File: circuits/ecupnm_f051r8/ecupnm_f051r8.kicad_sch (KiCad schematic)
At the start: 57 parts, among them J1 Conn_01x03_Pin, J2 Conn_01x03_Pin, J3 Conn_01x05_Pin, J4 Conn_01x03_Pin, J5 USB_B_Mini, U1 STM32F051R8Tx, U6 AMS1117-5.0, U7 AMS1117-3.3

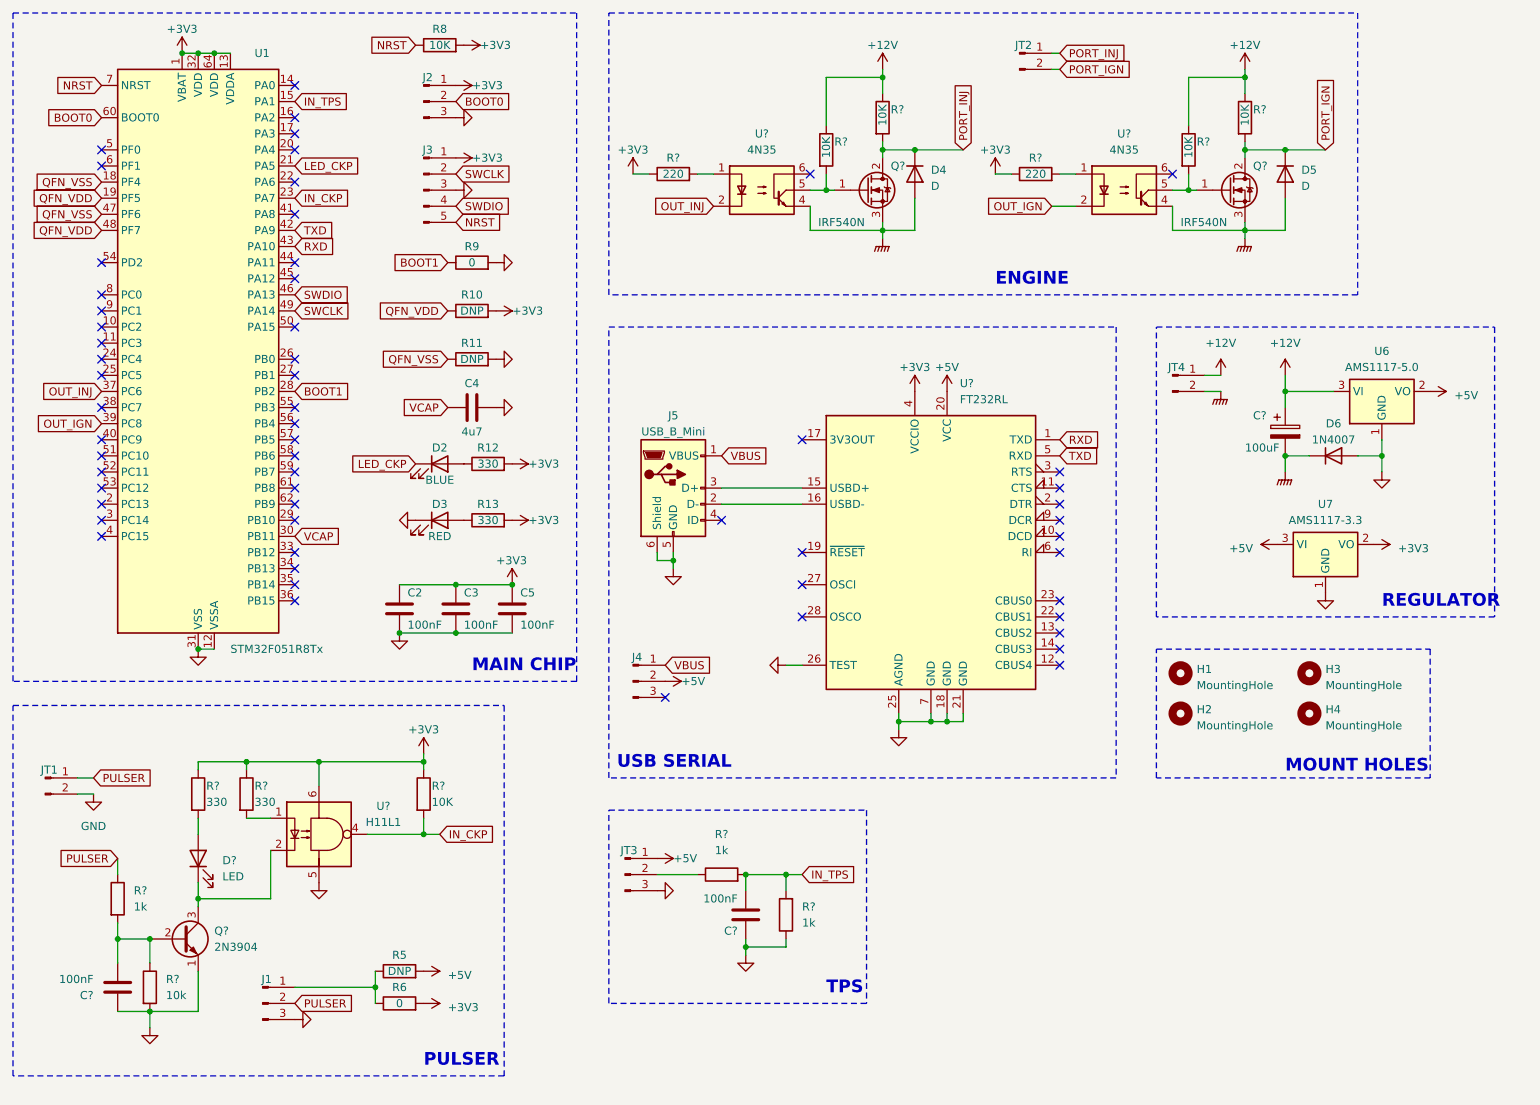
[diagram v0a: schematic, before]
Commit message: New PCB
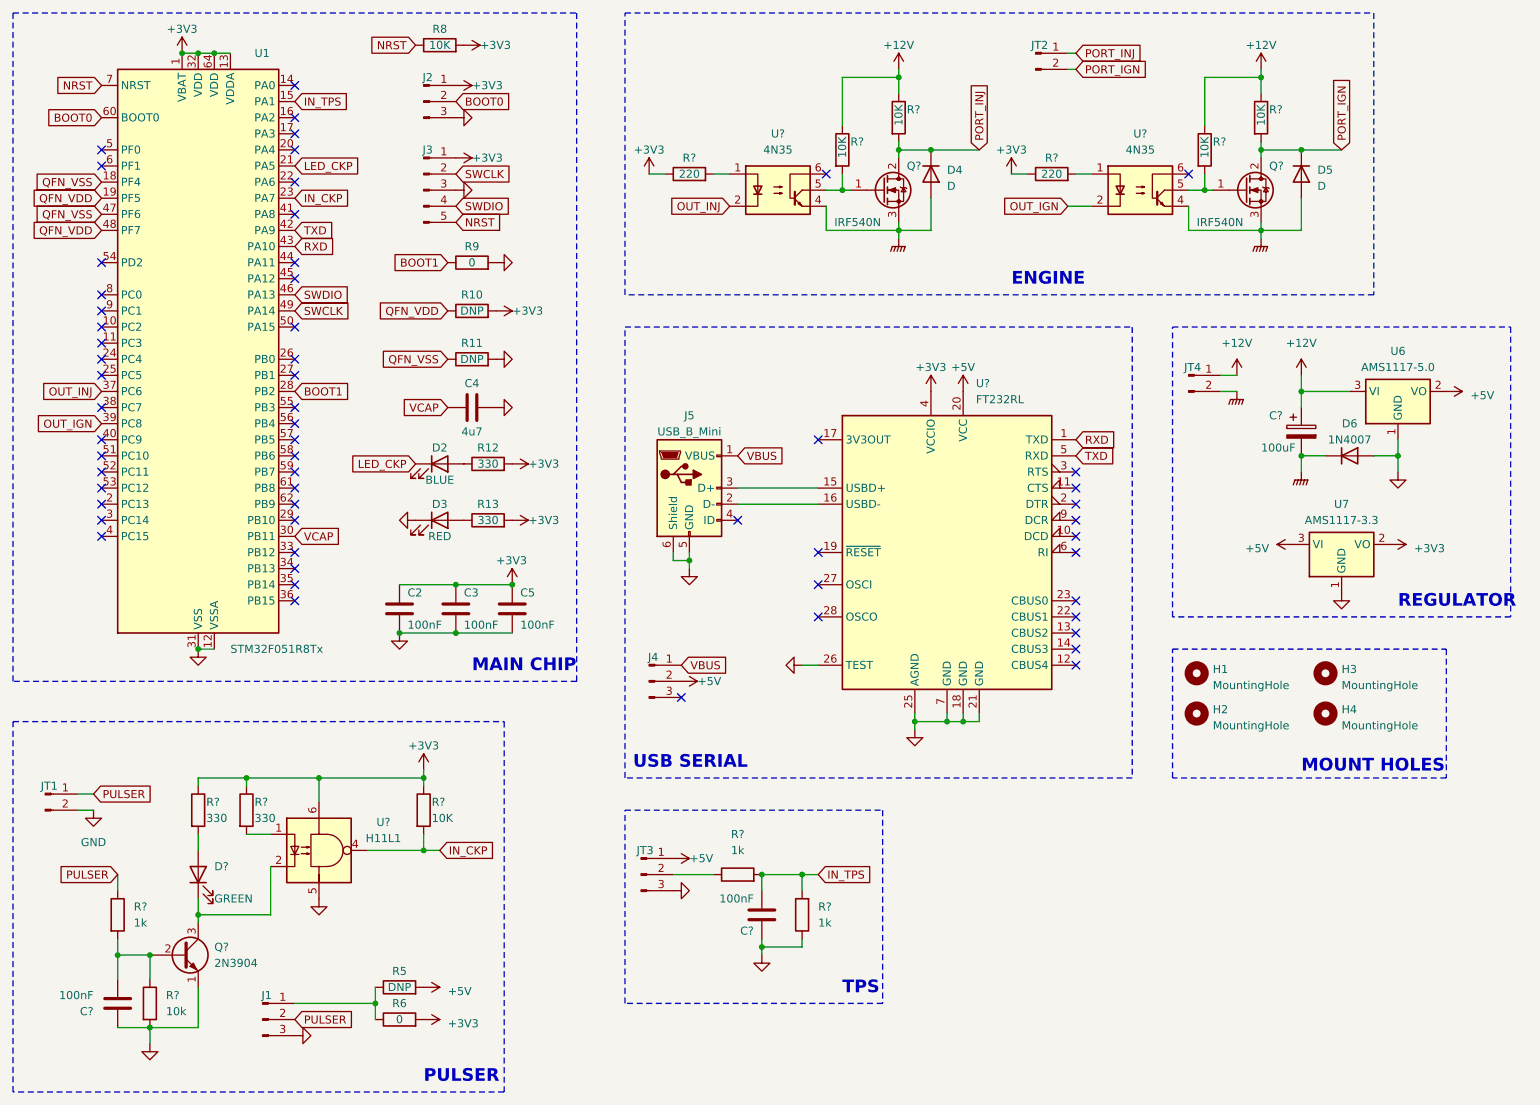
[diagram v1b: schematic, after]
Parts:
- C2, C3, C4, C5: footprint (none) -> Capacitor_SMD:C_0805_2012Metric_Pad1.18x1.45mm_HandSolder
- C? (x2): footprint Capacitor_SMD:C_1206_3216Metric_Pad1.33x1.80mm_HandSolder -> Capacitor_SMD:C_0805_2012Metric_Pad1.18x1.45mm_HandSolder
- D2, D3: footprint (none) -> LED_SMD:LED_0805_2012Metric_Pad1.15x1.40mm_HandSolder
- D?: value LED -> GREEN; footprint LED_SMD:LED_1206_3216Metric_Pad1.42x1.75mm_HandSolder -> LED_SMD:LED_0805_2012Metric_Pad1.15x1.40mm_HandSolder
- J2, J4: footprint (none) -> Connector_PinHeader_2.54mm:PinHeader_1x03_P2.54mm_Vertical
- J3: footprint (none) -> Connector_PinHeader_2.54mm:PinHeader_1x05_P2.54mm_Vertical
- R10, R11, R12, R13, R5, R6, R8, R9: footprint (none) -> Resistor_SMD:R_0805_2012Metric_Pad1.20x1.40mm_HandSolder
- R? (x13): footprint Resistor_SMD:R_1206_3216Metric_Pad1.30x1.75mm_HandSolder -> Resistor_SMD:R_0805_2012Metric_Pad1.20x1.40mm_HandSolder
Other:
- company: (none) -> Politeknik Negeri Madiun
- title: (none) -> Custom Engine Control
- moved on the sheet: C?, D4, D5, D6, D?, H1, H2, H3, H4, J1, J4, J5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

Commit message: PCB Baru
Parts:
- C?: footprint Capacitor_THT:CP_Radial_D7.5mm_P2.50mm -> Capacitor_THT:CP_Radial_D4.0mm_P2.00mm
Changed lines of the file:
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@@
       (effects (font (size 1.27 1.27)) (justify left))
     )
-    (property "Footprint" "Capacitor_THT:CP_Radial_D7.5mm_P2.50mm" (at 239.7252 90.17 0)
+    (property "Footprint" "Capacitor_THT:CP_Radial_D4.0mm_P2.00mm" (at 239.7252 90.17 0)
       (effects (font (size 1.27 1.27)) hide)
     )

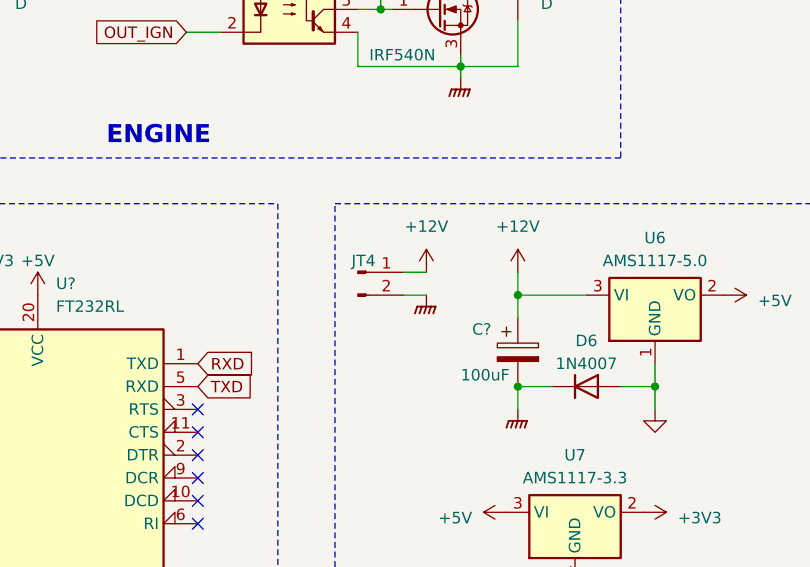
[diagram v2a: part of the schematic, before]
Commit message: Mulai Order
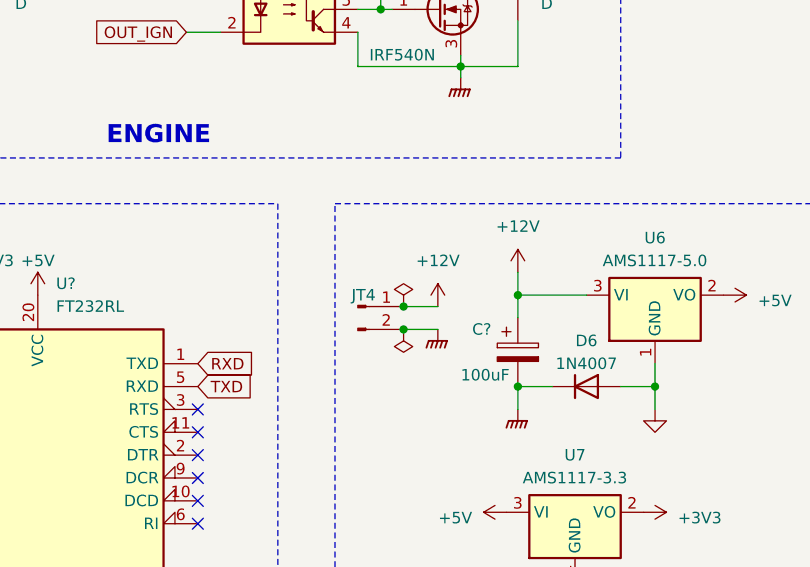
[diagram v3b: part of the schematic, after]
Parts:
- Q? (x2): footprint Package_TO_SOT_THT:TO-220-3_Horizontal_TabDown -> Package_TO_SOT_THT:TO-220-3_Vertical
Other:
- moved on the sheet: JT4
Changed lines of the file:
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@@
   (junction (at 177.8 132.08) (diameter 0) (color 0 0 0 0)
   )
+  (junction (at 226.06 81.28) (diameter 0) (color 0 0 0 0)
+  )
   (junction (at 72.39 140.97) (diameter 0) (color 0 0 0 0)
   )
@@
   (junction (at 96.52 118.11) (diameter 0) (color 0 0 0 0)
   )
+  (junction (at 226.06 83.82) (diameter 0) (color 0 0 0 0)
+  )
   (junction (at 153.67 167.64) (diameter 0) (color 0 0 0 0)
   )
@@
     (stroke (width 0) (type default))
   )
-  (wire (pts (xy 226.06 77.47) (xy 228.6 77.47))
+  (wire (pts (xy 226.06 81.28) (xy 229.87 81.28))
     (stroke (width 0) (type default))
   )
@@
     (stroke (width 0) (type default))
   )
-  (wire (pts (xy 226.06 80.01) (xy 228.6 80.01))
+  (wire (pts (xy 226.06 83.82) (xy 229.87 83.82))
     (stroke (width 0) (type default))
   )
@@
     )
   )
-  (symbol (lib_id "Connector:Conn_01x02_Pin") (at 220.98 77.47 0) (unit 1)
+  (symbol (lib_id "Connector:Conn_01x02_Pin") (at 220.98 81.28 0) (unit 1)
     (in_bom yes) (on_board yes) (dnp no) (fields_autoplaced)
-    (property "Reference" "JT4" (at 221.615 76.2 0)
+    (property "Reference" "JT4" (at 221.615 80.01 0)
       (effects (font (size 1.27 1.27)))
     )
-    (property "Value" "Conn_01x02_Pin" (at 221.615 76.2 0)
+    (property "Value" "Conn_01x02_Pin" (at 221.615 80.01 0)
       (effects (font (size 1.27 1.27)) hide)
     )
-    (property "Footprint" "TerminalBlock:TerminalBlock_Altech_AK300-2_P5.00mm" (at 220.98 77.47 0)
+    (property "Footprint" "TerminalBlock:TerminalBlock_Altech_AK300-2_P5.00mm" (at 220.98 81.28 0)
       (effects (font (size 1.27 1.27)) hide)
     )
-    (property "Datasheet" "~" (at 220.98 77.47 0)
+    (property "Datasheet" "~" (at 220.98 81.28 0)
       (effects (font (size 1.27 1.27)) hide)
     )
@@
       (effects (font (size 1.27 1.27)) (justify left))
     )
-    (property "Footprint" "Package_TO_SOT_THT:TO-220-3_Horizontal_TabDown" (at 179.07 50.165 0)
+    (property "Footprint" "Package_TO_SOT_THT:TO-220-3_Vertical" (at 179.07 50.165 0)
       (effects (font (size 1.27 1.27) italic) (justify left) hide)
     )
@@
     )
   )
-  (symbol (lib_id "power:+12V") (at 228.6 77.47 0) (unit 1)
+  (symbol (lib_id "power:+12V") (at 229.87 81.28 0) (unit 1)
     (in_bom yes) (on_board yes) (dnp no) (fields_autoplaced)
-    (property "Reference" "#PWR?" (at 228.6 81.28 0)
+    (property "Reference" "#PWR?" (at 229.87 85.09 0)
       (effects (font (size 1.27 1.27)) hide)
     )
-    (property "Value" "+12V" (at 228.6 72.39 0)
+    (property "Value" "+12V" (at 229.87 76.2 0)
       (effects (font (size 1.27 1.27)))
     )
-    (property "Footprint" "" (at 228.6 77.47 0)
+    (property "Footprint" "" (at 229.87 81.28 0)
       (effects (font (size 1.27 1.27)) hide)
     )
-    (property "Datasheet" "" (at 228.6 77.47 0)
+    (property "Datasheet" "" (at 229.87 81.28 0)
       (effects (font (size 1.27 1.27)) hide)
     )
@@
     )
   )
-  (symbol (lib_name "+12V_1") (lib_id "power:+12V") (at 175.26 29.21 0) (unit 1)
+  (symbol (lib_id "power:PWR_FLAG") (at 226.06 81.28 0) (unit 1)
+    (in_bom yes) (on_board yes) (dnp no) (fields_autoplaced)
+    (property "Reference" "#FLG01" (at 226.06 79.375 0)
+      (effects (font (size 1.27 1.27)) hide)
+    )
+    (property "Value" "PWR_FLAG" (at 226.06 77.47 0)
+      (effects (font (size 1.27 1.27)) hide)
+    )
+    (property "Footprint" "" (at 226.06 81.28 0)
+      (effects (font (size 1.27 1.27)) hide)
+    )
+    (property "Datasheet" "~" (at 226.06 81.28 0)
+      (effects (font (size 1.27 1.27)) hide)
+    )
+    (pin "1")
+    (instances
+      (project "ecupnm_f051r8"
+        (path "/6d87dde5-b75c-4573-a03b-3b31eef01557"
+          (reference "#FLG01") (unit 1)
+        )
+      )
+    )
+  )
+  (symbol (lib_id "power:+12V") (at 175.26 29.21 0) (unit 1)
     (in_bom yes) (on_board yes) (dnp no)
     (property "Reference" "#PWR028" (at 175.26 33.02 0)
@@
     )
   )
-  (symbol (lib_id "power:GNDPWR") (at 228.6 80.01 0) (unit 1)
+  (symbol (lib_id "power:GNDPWR") (at 229.87 83.82 0) (unit 1)
     (in_bom yes) (on_board yes) (dnp no) (fields_autoplaced)
-    (property "Reference" "#PWR?" (at 228.6 85.09 0)
+    (property "Reference" "#PWR?" (at 229.87 88.9 0)
       (effects (font (size 1.27 1.27)) hide)
     )
-    (property "Value" "GNDPWR" (at 228.473 85.09 0)
+    (property "Value" "GNDPWR" (at 229.743 88.9 0)
       (effects (font (size 1.27 1.27)) hide)
     )
-    (property "Footprint" "" (at 228.6 81.28 0)
+    (property "Footprint" "" (at 229.87 85.09 0)
       (effects (font (size 1.27 1.27)) hide)
     )
-    (property "Datasheet" "" (at 228.6 81.28 0)
+    (property "Datasheet" "" (at 229.87 85.09 0)
       (effects (font (size 1.27 1.27)) hide)
     )
@@
     )
   )
-  (symbol (lib_name "+12V_1") (lib_id "power:+12V") (at 232.41 29.21 0) (unit 1)
+  (symbol (lib_id "power:+12V") (at 232.41 29.21 0) (unit 1)
     (in_bom yes) (on_board yes) (dnp no)
     (property "Reference" "#PWR034" (at 232.41 33.02 0)
@@
       (effects (font (size 1.27 1.27)) (justify left))
     )
-    (property "Footprint" "Package_TO_SOT_THT:TO-220-3_Horizontal_TabDown" (at 236.22 50.165 0)
+    (property "Footprint" "Package_TO_SOT_THT:TO-220-3_Vertical" (at 236.22 50.165 0)
       (effects (font (size 1.27 1.27) italic) (justify left) hide)
     )
@@
         )
       )
+    )
+  )
+  (symbol (lib_id "power:PWR_FLAG") (at 226.06 83.82 180) (unit 1)
+    (in_bom yes) (on_board yes) (dnp no) (fields_autoplaced)
+    (property "Reference" "#FLG02" (at 226.06 85.725 0)
+      (effects (font (size 1.27 1.27)) hide)
+    )
+    (property "Value" "PWR_FLAG" (at 226.06 87.63 0)
+      (effects (font (size 1.27 1.27)) hide)
+    )
+    (property "Footprint" "" (at 226.06 83.82 0)
+      (effects (font (size 1.27 1.27)) hide)
+    )
+    (property "Datasheet" "~" (at 226.06 83.82 0)
+      (effects (font (size 1.27 1.27)) hide)
+    )
+    (pin "1")
+    (instances
+      (project "ecupnm_f051r8"
+        (path "/6d87dde5-b75c-4573-a03b-3b31eef01557"
+          (reference "#FLG02") (unit 1)
+        )
+      )
